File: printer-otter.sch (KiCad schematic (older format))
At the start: 49 parts, among them J1 USB, J2 Printer, J4 Encoder, J5 UART, J6 Analog, Q1 Q_NMOS_GSD, Q2 Q_PMOS_GSD, Q3 Q_NMOS_GSD, Q4 Q_PMOS_GSD, SW1 Down, U1 MT3608, U2 STM32F072C8Ux, U3 AP2204R-3.3, U4 USBLC6-4SC6, U5 L78L09_SOT89, U6 4504, U7 4504

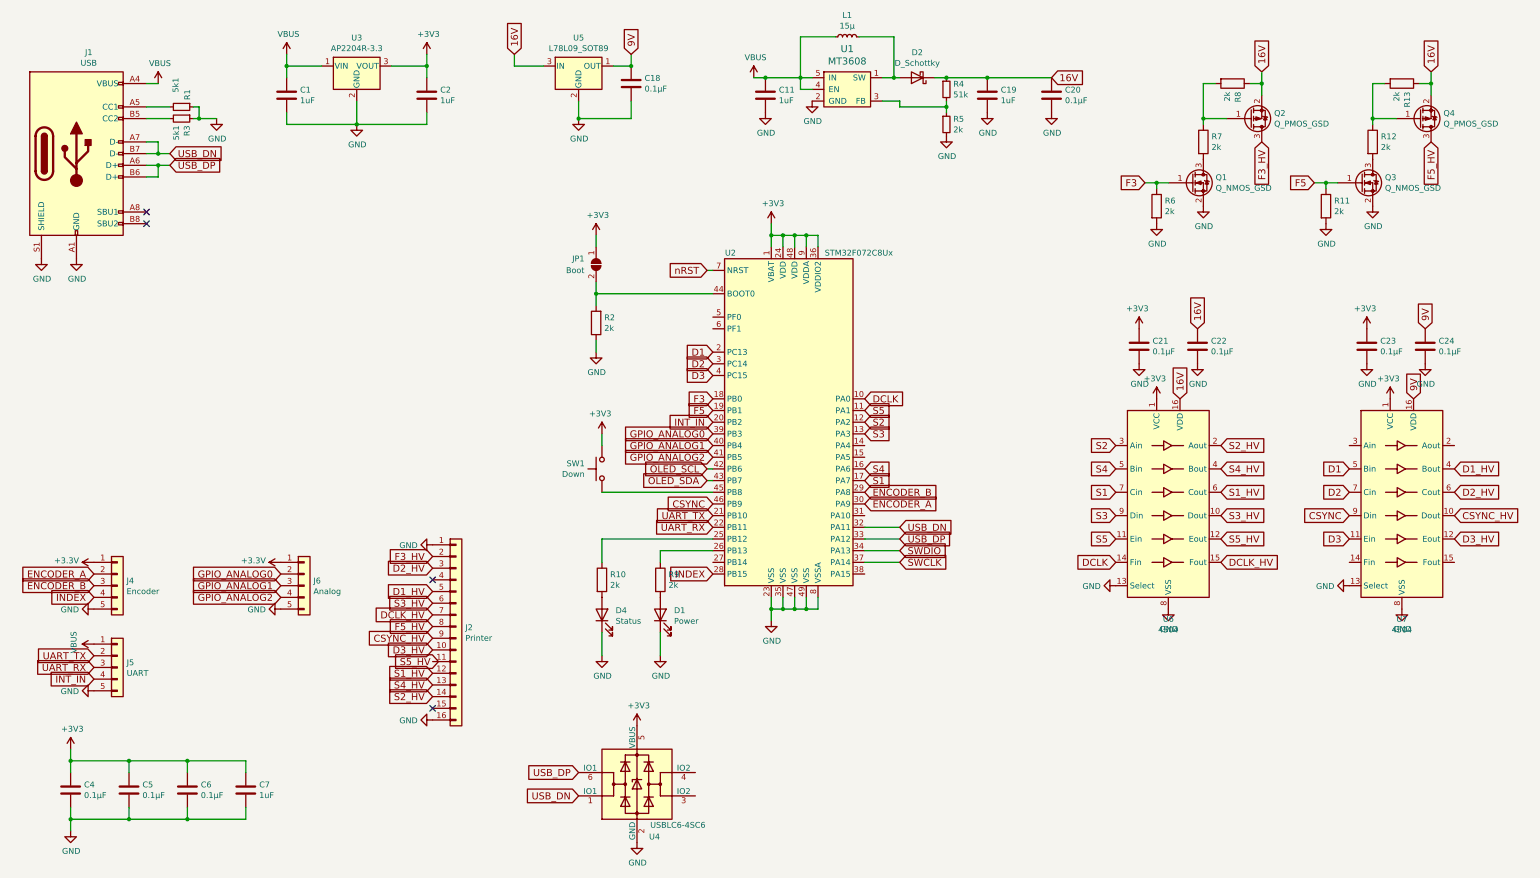
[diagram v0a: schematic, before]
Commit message: schematic cleanup
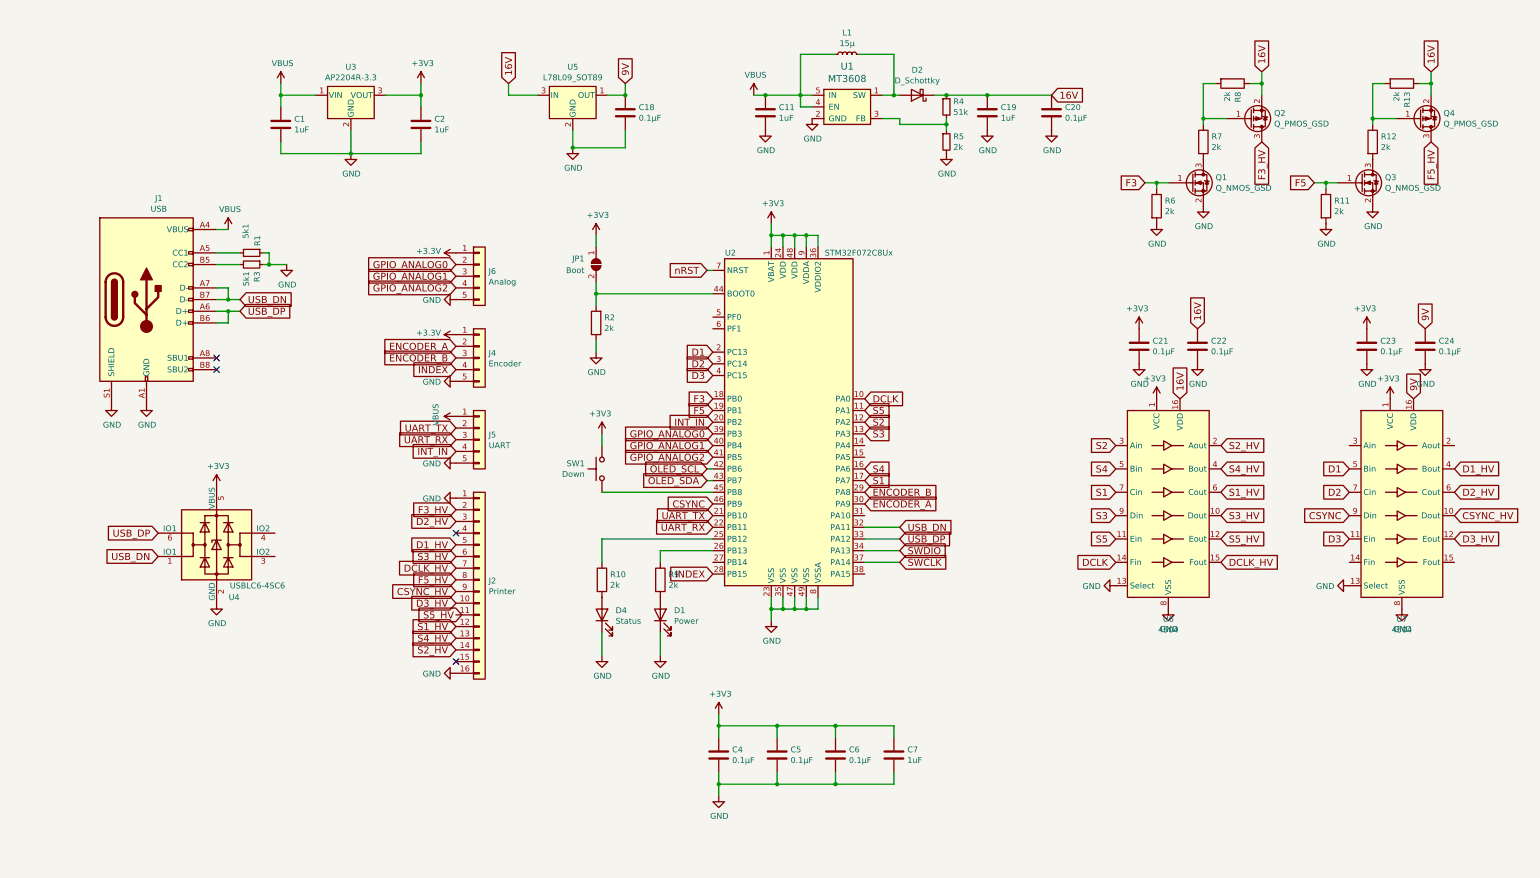
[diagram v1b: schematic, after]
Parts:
- U6, U7: footprint Package_SO:SOIC-16W_5.3x10.2mm_P1.27mm -> Package_SO:SOIC-16_3.9x9.9mm_P1.27mm
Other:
- moved on the sheet: C1, C11, C18, C19, C2, C20, C4, C5, C6, C7, D2, J1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
